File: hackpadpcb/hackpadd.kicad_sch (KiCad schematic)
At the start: 9 parts, among them SW1 SW_Push, SW2 SW_Push, SW3 SW_Push, SW4 SW_Push, SW5 RotaryEncoder, SW6 SW_Push, SW7 SW_Push, U1 XIAO-RP2040-DIP

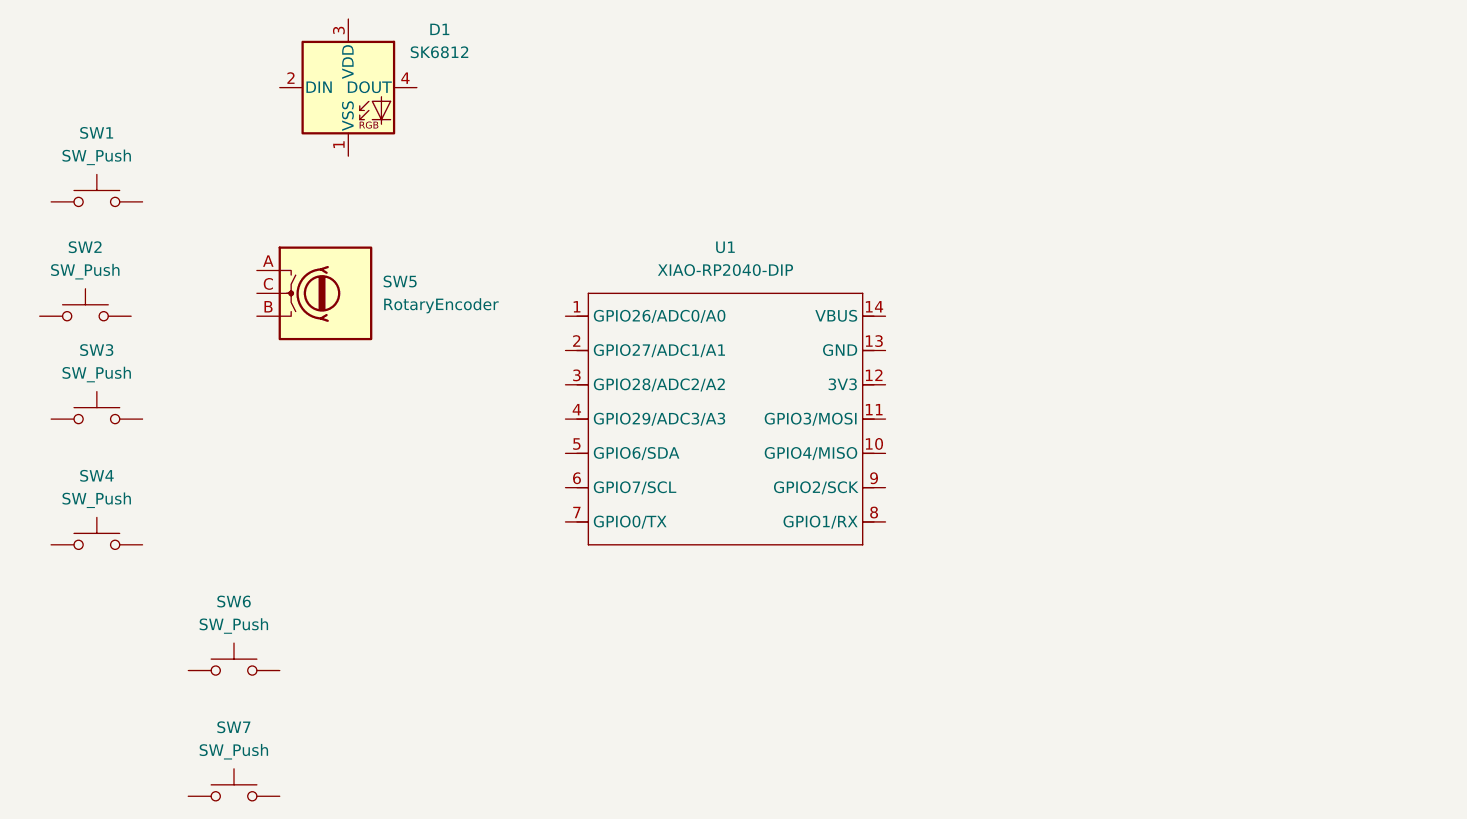
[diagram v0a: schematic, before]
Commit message: finish schem and pcb
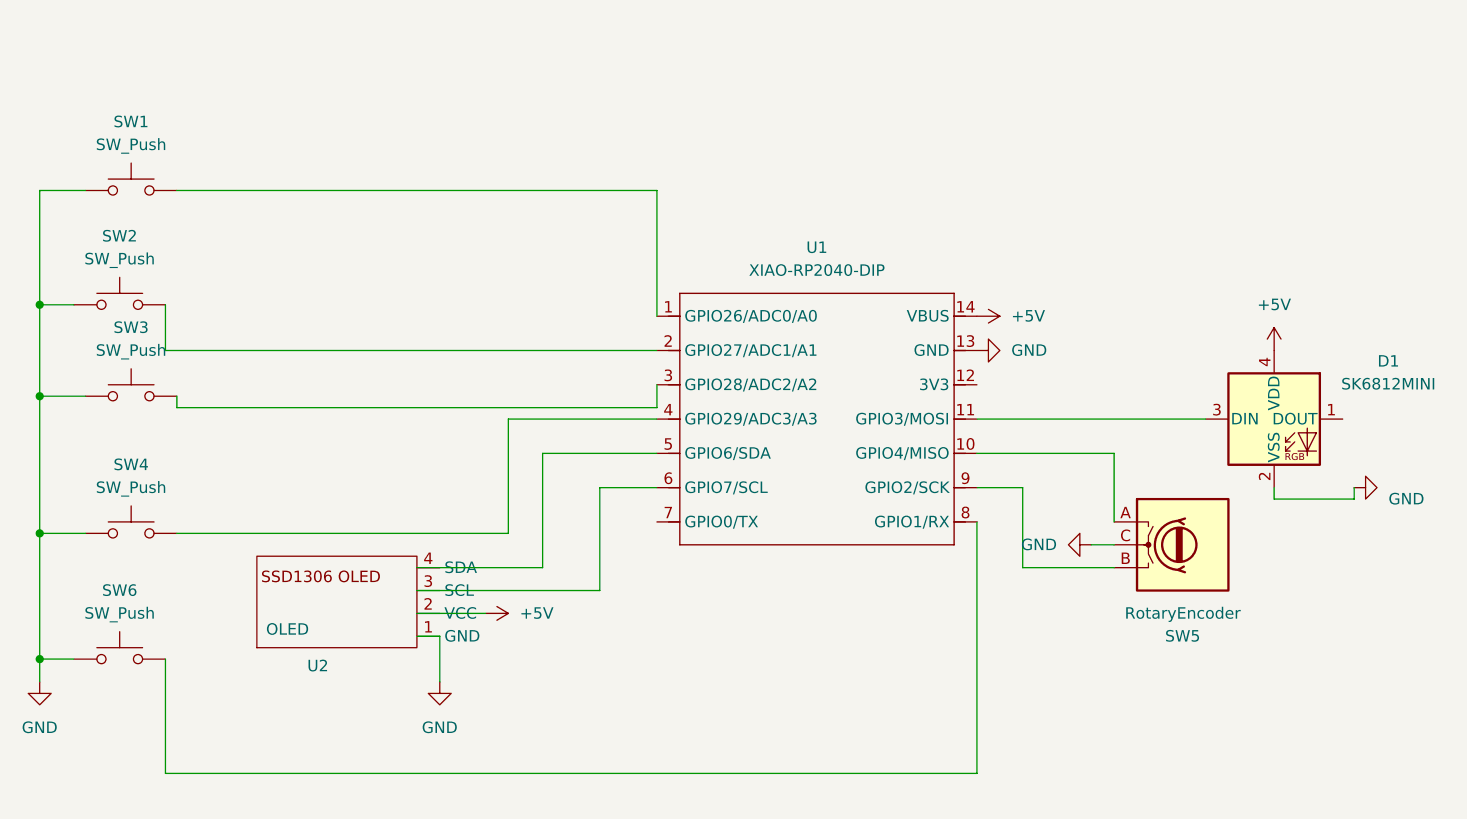
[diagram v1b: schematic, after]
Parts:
- removed D1: SK6812, LED_SMD:LED_SK6812_PLCC4_5.0x5.0mm_P3.2mm, symbol LED:SK6812
- removed SW7: SW_Push, symbol Switch:SW_Push
- added D1: SK6812MINI, LED_SMD:LED_SK6812MINI_PLCC4_3.5x3.5mm_P1.75mm, symbol LED:SK6812MINI
- added U2: OLED, OLED:SSD1306-0.91-OLED-4pin-128x32 (1), symbol oled:oled_symb
- SW1, SW2, SW3, SW4, SW6: footprint (none) -> Button_Switch_Keyboard:SW_Cherry_MX_1.00u_PCB
- SW5: footprint (none) -> Rotary_Encoder:RotaryEncoder_Alps_EC11E_Vertical_H20mm
- U1: footprint Module:MOUDLE14P-XIAO-DIP-SMD -> OPL:XIAO-RP2040-DIP
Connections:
- net GND: now reaches SW2.1
- net GND: now also SW1.1, SW3.1, SW4.1, SW5.C, SW6.1, U1.13 (GND), D1.2 (VSS), U2.1 (GND)
- net at SW2.2: now also U1.2 (GPIO27/ADC1/A1)
- net at SW3.2: now also U1.3 (GPIO28/ADC2/A2)
- net at SW5.A: now also U1.10 (GPIO4/MISO)
- net at SW5.B: now also U1.9 (GPIO2/SCK)
- net at U1.1 (GPIO26/ADC0/A0): now also SW1.2
- net at U1.11 (GPIO3/MOSI): now also D1.3 (DIN)
- net +5V: now reaches U1.14 (VBUS)
- net +5V: now also D1.4 (VDD), U2.2 (VCC)
- net at U1.4 (GPIO29/ADC3/A3): now also SW4.2
- net at U1.5 (GPIO6/SDA): now also U2.4 (SDA)
- net at U1.6 (GPIO7/SCL): now also U2.3 (SCL)
- net at U1.8 (GPIO1/RX): now also SW6.2
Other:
- moved on the sheet: SW1, SW2, SW3, SW4, SW5, U1
